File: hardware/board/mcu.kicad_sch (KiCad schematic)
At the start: 25 parts, among them J10 Dotstars, J11 USB, J2 SWD, J3 USB B, SW2 Reset, U5 ATSAMD51J20A-M, Y1 32.768 kHz

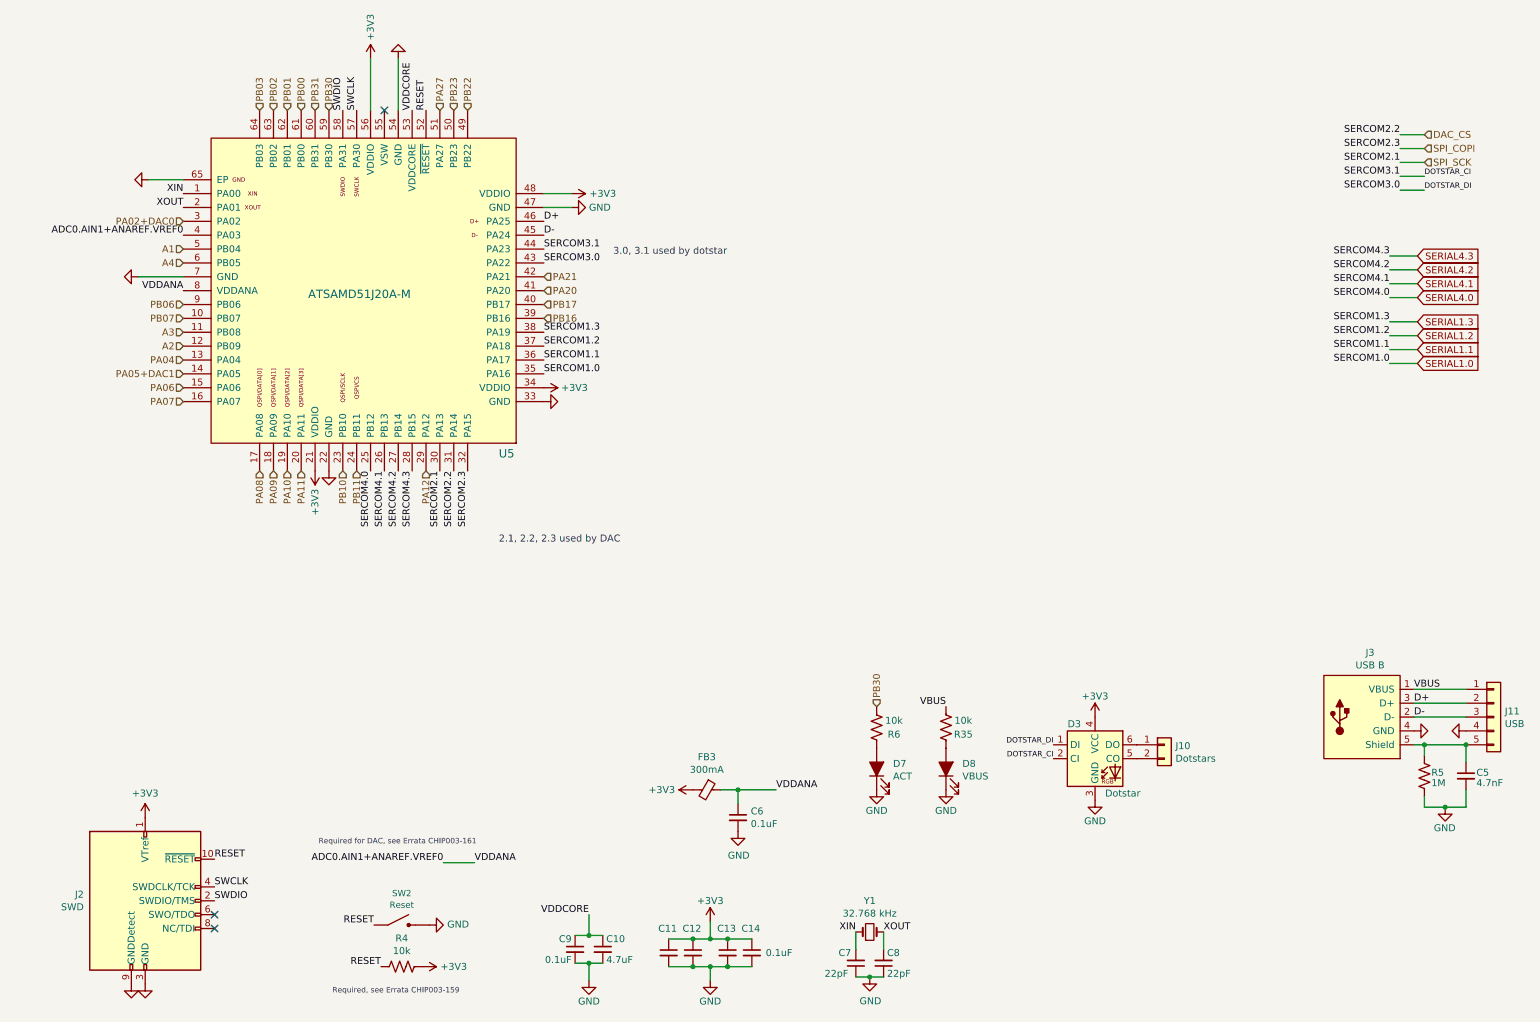
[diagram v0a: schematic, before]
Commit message: Initial stab at hardware revision
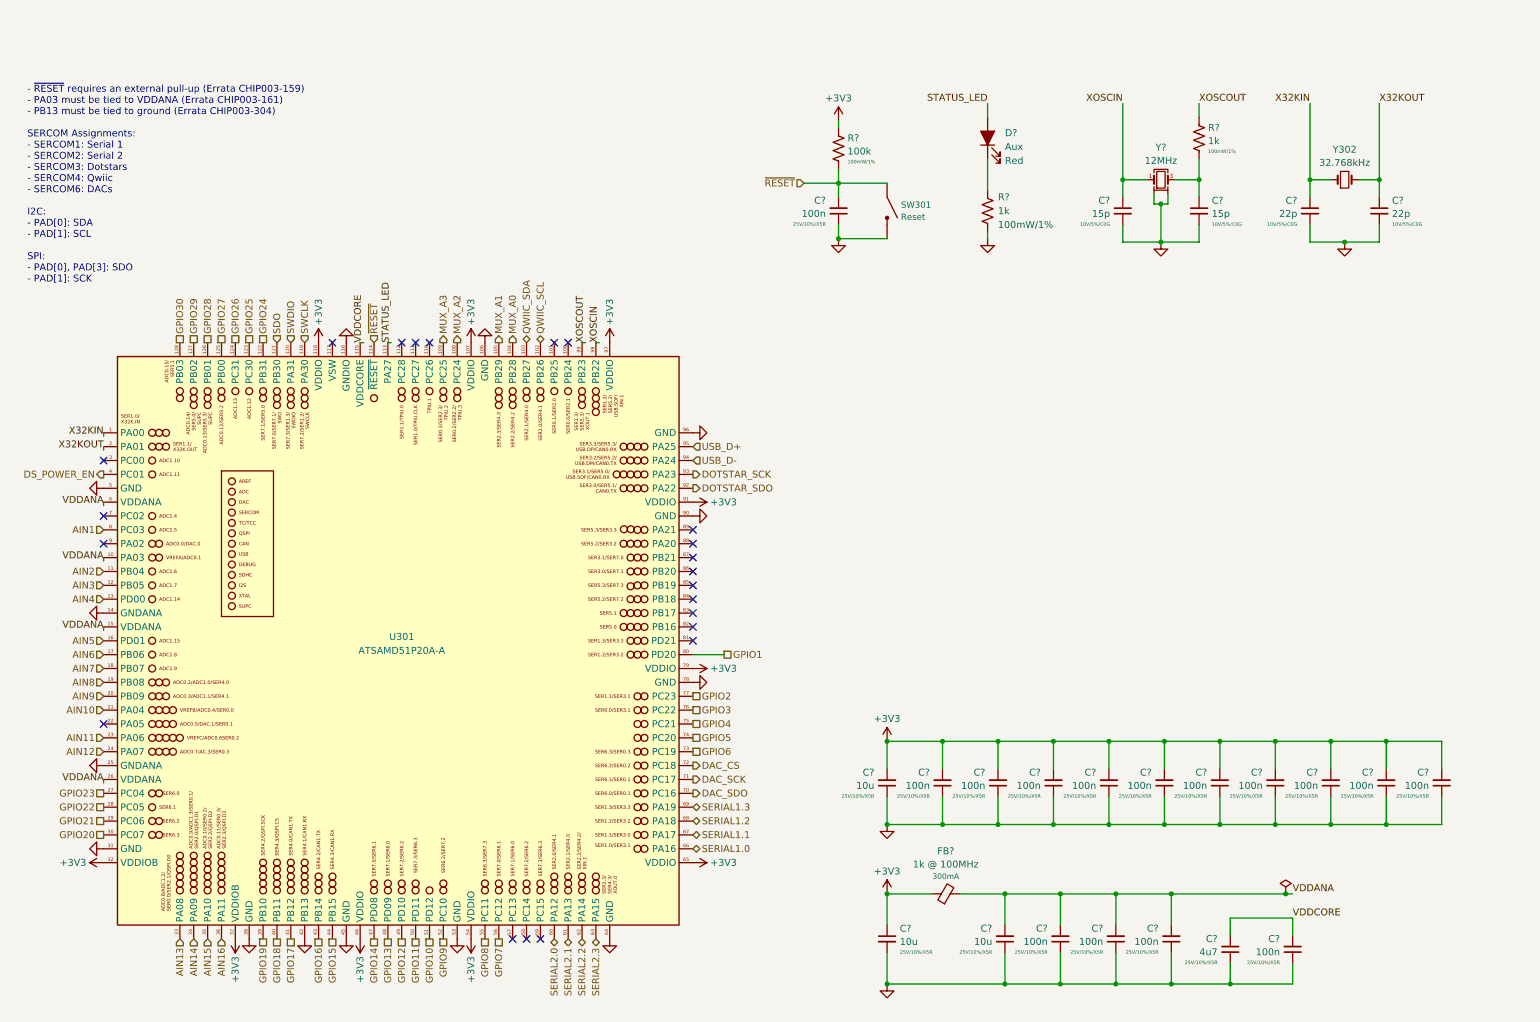
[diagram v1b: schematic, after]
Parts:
- removed C10: 4.7uF, Capacitor_SMD:C_0603_1608Metric_Pad1.08x0.95mm_HandSolder, symbol Device:C_Small
- removed C11, C12, C13, C14, C6, C9: 0.1uF, Capacitor_SMD:C_0603_1608Metric_Pad1.08x0.95mm_HandSolder, symbol Device:C_Small
- removed C5: 4.7nF, Capacitor_SMD:C_0603_1608Metric_Pad1.08x0.95mm_HandSolder, symbol Device:C_Small
- removed C7, C8: 22pF, Capacitor_SMD:C_0603_1608Metric_Pad1.08x0.95mm_HandSolder, symbol Device:C_Small
- removed D3: Dotstar, winterbloom:Dotstar_5050, symbol winterbloom:Dotstar
- removed D7: ACT, winterbloom:LED_0805_Kingbright_APT2012, symbol Device:LED_ALT
- removed D8: VBUS, winterbloom:LED_0805_Kingbright_APT2012, symbol Device:LED_ALT
- removed FB3: 300mA, Inductor_SMD:L_0603_1608Metric_Pad1.05x0.95mm_HandSolder, symbol Device:Ferrite_Bead_Small
- removed J10: Dotstars, Connector_PinHeader_2.54mm:PinHeader_1x02_P2.54mm_Vertical, symbol Connector_Generic:Conn_01x02
- removed J11: USB, Connector_PinHeader_2.54mm:PinHeader_1x05_P2.54mm_Vertical, symbol Connector_Generic:Conn_01x05
- removed J2: SWD, Connector_PinHeader_1.27mm:PinHeader_2x05_P1.27mm_Vertical, symbol Connector:Conn_ARM_JTAG_SWD_10
- removed J3: USB B, Connector_USB:USB_B_OST_USB-B1HSxx_Horizontal, symbol winterbloom:USB_B_Receptacle
- removed R35, R4, R6: 10k, Resistor_SMD:R_0603_1608Metric_Pad0.98x0.95mm_HandSolder, symbol Device:R_US
- removed R5: 1M, Resistor_SMD:R_0805_2012Metric_Pad1.20x1.40mm_HandSolder, symbol Device:R_US
- removed SW2: Reset, winterbloom:Tactile_Switch_4.2mm, symbol winterbloom:Tactile_Switch
- removed U5: ATSAMD51J20A-M, winterbloom:QFN+QFP-64-SAMD51, symbol winterbloom:ATSAMD51J20A-M
- added C? (x3): 10u, winterbloom:C_0805_HandSolder, symbol Device:C_Small
- added C? (x15): 100n, winterbloom:C_0603_HandSolder, symbol Device:C_Small
- added C? (x2): 22p, winterbloom:C_0603_HandSolder, symbol Device:C_Small
- added C? (x2): 15p, winterbloom:C_0603_HandSolder, symbol Device:C_Small
- added C?: 4u7, winterbloom:C_0603_HandSolder, symbol Device:C_Small
- added D?: Aux, winterbloom:LED_0805_Kingbright_APT2012, symbol Device:LED_Filled
- added FB?: 1k @ 100MHz, winterbloom:L_0603_HandSolder, symbol Device:FerriteBead_Small
- added R? (x2): 1k, winterbloom:R_0603_HandSolder, symbol Device:R_US
- added R?: 100k, winterbloom:R_0603_HandSolder, symbol Device:R_US
- added SW301: Reset, winterbloom:Tactile_Switch_4.2mm, symbol winterbloom:Tactile_Switch
- added U301: ATSAMD51P20A-A, Package_QFP:TQFP-128_14x14mm_P0.4mm, symbol winterbloom:ATSAMD51P20A-A
- added Y?: 12MHz, Crystal:Crystal_SMD_Abracon_ABM8G-4Pin_3.2x2.5mm, symbol winterbloom:Crystal_12MHz_4Pin
- Y302: renamed from Y1; value 32.768 kHz -> 32.768kHz
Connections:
- net +3V3: now also C?.1, C?.2, C?.2, C?.2, C?.2, C?.2, C?.2, C?.2, C?.2, C?.2, C?.2, C?.2, FB?.1, R?.1, U301.107 (VDDIO), U301.118 (VDDIO), U301.32 (VDDIOB), U301.37 (VDDIOB), U301.46 (VDDIO), U301.54 (VDDIO), U301.65 (VDDIO), U301.79 (VDDIO), U301.91 (VDDIO), U301.97 (VDDIO)
- net DAC_CS: now also U301.72 (PC18)
- net GND: now also C?.1, C?.1, C?.1, C?.1, C?.1, C?.1, C?.1, C?.1, C?.1, C?.1, C?.1, C?.1, C?.1, C?.1, C?.1, C?.1, C?.1, C?.1, C?.2, C?.2, C?.2, C?.2, C?.2, R?.2, SW301.2, U301.106 (GND), U301.116 (GNDIO), U301.14 (GNDANA), U301.25 (GNDANA), U301.31 (GND), U301.38 (GND), U301.42 (PB13), U301.45 (GND), U301.5 (GND), U301.53 (GND), U301.64 (GND), U301.78 (GND), U301.90 (GND), U301.96 (GND), Y?.2, Y?.4
- net SERIAL1.0: now also U301.66 (PA16)
- net SERIAL1.1: now also U301.67 (PA17)
- net SERIAL1.2: now also U301.68 (PA18)
- net SERIAL1.3: now also U301.69 (PA19)
- net SWCLK: now also U301.119 (PA30)
- net SWDIO: now also U301.120 (PA31)
- net VDDCORE: now also C?.2, C?.2, U301.115 (VDDCORE)
- net XIN renamed X32KIN
- net X32KIN: now also C?.1, U301.1 (PA00)
- net XOUT renamed X32KOUT
- net X32KOUT: now also C?.1, U301.2 (PA01)
- new net: C?.1, R?.2, Y?.3
- new net: D?.1 (K), R?.1
- new net AIN1: U301.8 (PC03)
- new net AIN10: U301.21 (PA04)
- new net AIN11: U301.23 (PA06)
- new net AIN12: U301.24 (PA07)
- new net AIN13: U301.33 (PA08)
- new net AIN14: U301.34 (PA09)
- new net AIN15: U301.35 (PA10)
- new net AIN16: U301.36 (PA11)
- new net AIN2: U301.11 (PB04)
- new net AIN3: U301.12 (PB05)
- new net AIN4: U301.13 (PD00)
- new net AIN5: U301.16 (PD01)
- new net AIN6: U301.17 (PB06)
- new net AIN7: U301.18 (PB07)
- new net AIN8: U301.19 (PB08)
- new net AIN9: U301.20 (PB09)
- new net DAC_SCK: U301.71 (PC17)
- new net DAC_SDO: U301.70 (PC16)
- new net DOTSTAR_SCK: U301.93 (PA23)
- new net DOTSTAR_SDO: U301.92 (PA22)
- new net DS_POWER_EN: U301.4 (PC01)
- new net GPIO1: U301.80 (PD20)
- new net GPIO10: U301.51 (PD12)
- new net GPIO11: U301.50 (PD11)
- new net GPIO12: U301.49 (PD10)
- new net GPIO13: U301.48 (PD09)
- new net GPIO14: U301.47 (PD08)
- new net GPIO15: U301.44 (PB15)
- new net GPIO16: U301.43 (PB14)
- new net GPIO17: U301.41 (PB12)
- new net GPIO18: U301.40 (PB11)
- new net GPIO19: U301.39 (PB10)
- new net GPIO2: U301.77 (PC23)
- new net GPIO20: U301.30 (PC07)
- new net GPIO21: U301.29 (PC06)
- new net GPIO22: U301.28 (PC05)
- new net GPIO23: U301.27 (PC04)
- new net GPIO24: U301.122 (PB31)
- new net GPIO25: U301.123 (PC30)
- new net GPIO26: U301.124 (PC31)
- new net GPIO27: U301.125 (PB00)
- new net GPIO28: U301.126 (PB01)
- new net GPIO29: U301.127 (PB02)
- new net GPIO3: U301.76 (PC22)
- new net GPIO30: U301.128 (PB03)
- new net GPIO4: U301.75 (PC21)
- new net GPIO5: U301.74 (PC20)
- new net GPIO6: U301.73 (PC19)
- new net GPIO7: U301.56 (PC12)
- new net GPIO8: U301.55 (PC11)
- new net GPIO9: U301.52 (PC10)
- new net MUX_A0: U301.104 (PB28)
- new net MUX_A1: U301.105 (PB29)
- new net MUX_A2: U301.108 (PC24)
- new net MUX_A3: U301.109 (PC25)
- new net QWIIC_SCL: U301.102 (PB26)
- new net QWIIC_SDA: U301.103 (PB27)
- new net SDO: U301.121 (PB30)
- new net SERIAL2.0: U301.60 (PA12)
- new net SERIAL2.1: U301.61 (PA13)
- new net SERIAL2.2: U301.62 (PA14)
- new net SERIAL2.3: U301.63 (PA15)
- new net STATUS_LED: D?.2 (A), U301.113 (PA27)
- new net USB_D+: U301.95 (PA25)
- new net USB_D-: U301.94 (PA24)
- new net VDDANA: C?.2, C?.2, C?.2, C?.2, FB?.2, U301.10 (PA03), U301.15 (VDDANA), U301.26 (VDDANA), U301.6 (VDDANA)
- new net XOSCIN: C?.1, U301.98 (PB22), Y?.1
- new net XOSCOUT: R?.1, U301.99 (PB23)
- new net ~{RESET}: C?.2, R?.2, SW301.1, U301.114 (~{RESET})
- no-connect marks 3 -> 22
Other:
- note added: "- ~{RESET} requires an external pull-up (Errata CHIP003-159) - PA03 must be tied to VDDANA (Errata CHIP003-161) - PB13 must be tied to ground (Errata CHIP003-304) SERCOM Assignments: - SERCOM1: Serial 1 - SERCOM2: Serial 2 - SERCOM3: Dotstars - SERCOM4: Qwiic - SERCOM6: DACs I2C: - PAD[0]: SDA - PAD[1]: SCL SPI: - PAD[0], PAD[3]: SDO - PAD[1]: SCK"
- note removed: "2.1, 2.2, 2.3 used by DAC"
- note removed: "3.0, 3.1 used by dotstar"
- note removed: "Required for DAC, see Errata CHIP003-161"
- note removed: "Required, see Errata CHIP003-159"
- moved on the sheet: Y302
